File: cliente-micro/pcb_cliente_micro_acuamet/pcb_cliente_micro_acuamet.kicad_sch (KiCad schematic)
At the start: 43 parts, among them J1 Presion, J10 5V IN, J11 Botones, J2 Ultrasonico, J3 Valvula 1, J4 Valvula 2, J5 Relay, J6 Debug, J7 Valvula 3, J8 LCD, J9 Valvula 4, U1 M7, U2 M7, U3 AMS1117-3.3_C347222, U4 ESP32-WROOM-32D

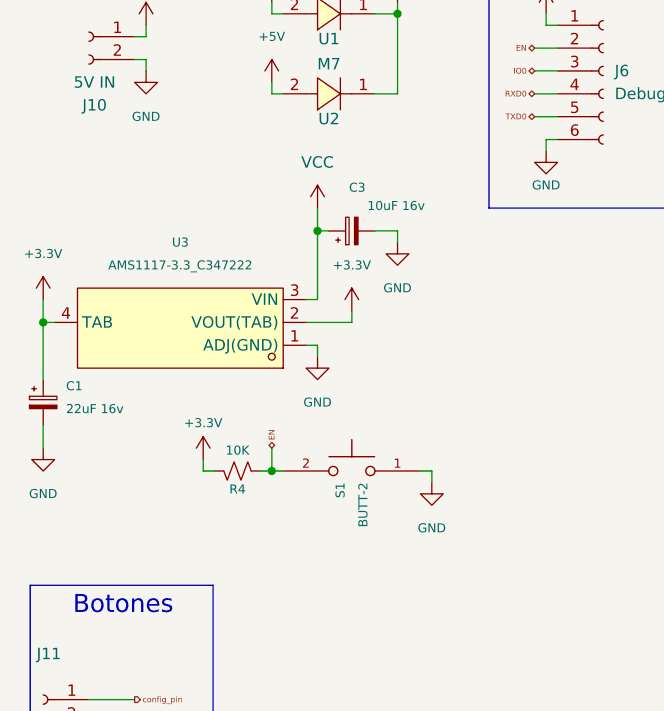
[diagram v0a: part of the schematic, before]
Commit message: Version final PCB
Version revisada y corregida
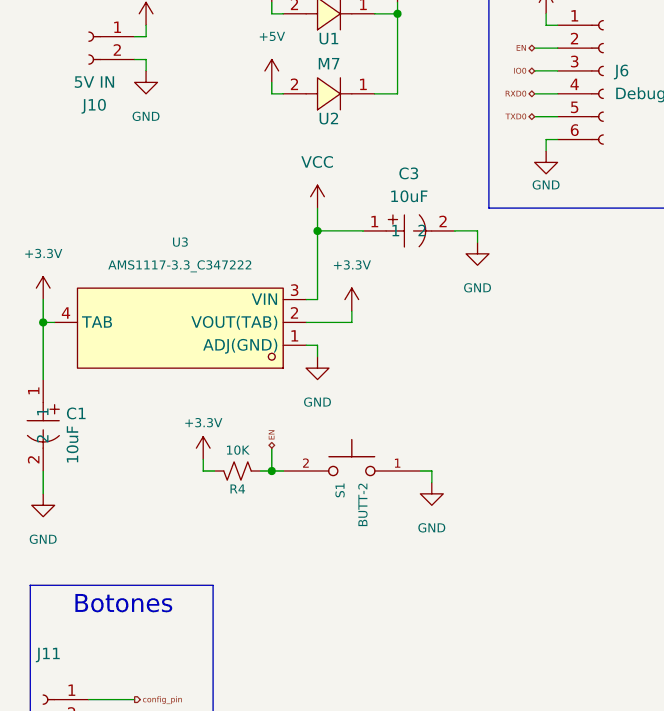
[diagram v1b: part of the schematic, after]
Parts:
- removed C1: 22uF 16v, Capacitor_THT:CP_Radial_D6.3mm_P2.50mm, symbol Device:C_Polarized_Small
- removed C3: 10uF 16v, Capacitor_THT:CP_Radial_D6.3mm_P2.50mm, symbol Device:C_Polarized_Small
- added C1, C3: 10uF, EasyEDA:CAP-SMD_L3.2-W1.6, symbol EasyEDA:TMCMA1C106KTRF
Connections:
- net +3.3V: now also C1.1
- net GND: now also C1.2, C3.2
- net VCC: now also C3.1
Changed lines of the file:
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@@
 	(wire
 		(pts
-			(xy 54.61 46.99) (xy 57.15 46.99)
+			(xy 63.5 46.99) (xy 66.04 46.99)
 		)
 		(stroke
@@
 	(wire
 		(pts
-			(xy 57.15 46.99) (xy 57.15 48.26)
+			(xy 66.04 46.99) (xy 66.04 48.26)
 		)
 		(stroke
@@
 	(wire
 		(pts
+			(xy 17.78 73.66) (xy 17.78 76.2)
+		)
+		(stroke
+			(width 0)
+			(type default)
+		)
+	)
+	(wire
+		(pts
 			(xy 91.44 26.67) (xy 91.44 25.4)
 		)
@@
 	(wire
 		(pts
-			(xy 17.78 68.58) (xy 17.78 71.12)
-		)
-		(stroke
-			(width 0)
-			(type default)
-		)
-	)
-	(wire
-		(pts
 			(xy 139.7 163.83) (xy 143.51 163.83)
 		)
@@
 	(wire
 		(pts
-			(xy 48.26 46.99) (xy 49.53 46.99)
+			(xy 48.26 46.99) (xy 53.34 46.99)
 		)
 		(stroke
@@
 	(symbol
 		(lib_id "power:GND")
-		(at 57.15 48.26 0)
+		(at 66.04 48.26 0)
 		(unit 1)
 		(exclude_from_sim no)
@@
 		(fields_autoplaced yes)
 		(property "Reference" "#PWR023"
-			(at 57.15 54.61 0)
+			(at 66.04 54.61 0)
 			(effects
 				(font
@@
 		)
 		(property "Value" "GND"
-			(at 57.15 53.34 0)
+			(at 66.04 53.34 0)
 			(effects
 				(font
@@
 		)
 		(property "Footprint" ""
-			(at 57.15 48.26 0)
+			(at 66.04 48.26 0)
 			(effects
 				(font
@@
 		)
 		(property "Datasheet" ""
-			(at 57.15 48.26 0)
+			(at 66.04 48.26 0)
 			(effects
 				(font
@@
 		)
 		(property "Description" "Power symbol creates a global label with name \"GND\" , ground"
-			(at 57.15 48.26 0)
+			(at 66.04 48.26 0)
 			(effects
 				(font
@@
 	)
 	(symbol
-		(lib_id "Device:C_Polarized_Small")
-		(at 52.07 46.99 90)
-		(unit 1)
-		(exclude_from_sim no)
-		(in_bom yes)
-		(on_board yes)
-		(dnp no)
-		(property "Reference" "C3"
-			(at 53.594 42.164 90)
-			(effects
-				(font
-					(size 1 1)
-				)
-				(justify left)
-			)
-		)
-		(property "Value" "10uF 16v"
-			(at 60.198 44.196 90)
-			(effects
-				(font
-					(size 1 1)
-				)
-				(justify left)
-			)
-		)
-		(property "Footprint" "Capacitor_THT:CP_Radial_D6.3mm_P2.50mm"
-			(at 52.07 46.99 0)
-			(effects
-				(font
-					(size 1.27 1.27)
-				)
-				(hide yes)
-			)
-		)
-		(property "Datasheet" "~"
-			(at 52.07 46.99 0)
-			(effects
-				(font
-					(size 1.27 1.27)
-				)
-				(hide yes)
-			)
-		)
-		(property "Description" "Polarized capacitor, small symbol"
-			(at 52.07 46.99 0)
-			(effects
-				(font
-					(size 1.27 1.27)
-				)
-				(hide yes)
-			)
-		)
-		(pin "1"
-		)
-		(pin "2"
-		)
-		(instances
-			(project ""
-				(path "/40156f8c-40d9-435e-851b-9df8dfaedb63"
-					(reference "C3")
-					(unit 1)
-				)
-			)
-		)
-	)
-	(symbol
 		(lib_id "power:+5V")
 		(at 43.18 30.48 0)
@@
 	(symbol
 		(lib_id "power:GND")
-		(at 17.78 71.12 0)
+		(at 17.78 76.2 0)
 		(unit 1)
 		(exclude_from_sim no)
@@
 		(fields_autoplaced yes)
 		(property "Reference" "#PWR04"
-			(at 17.78 77.47 0)
+			(at 17.78 82.55 0)
 			(effects
 				(font
@@
 		)
 		(property "Value" "GND"
-			(at 17.78 76.2 0)
+			(at 17.78 81.28 0)
 			(effects
 				(font
@@
 		)
 		(property "Footprint" ""
-			(at 17.78 71.12 0)
+			(at 17.78 76.2 0)
 			(effects
 				(font
@@
 		)
 		(property "Datasheet" ""
-			(at 17.78 71.12 0)
+			(at 17.78 76.2 0)
 			(effects
 				(font
@@
 		)
 		(property "Description" "Power symbol creates a global label with name \"GND\" , ground"
-			(at 17.78 71.12 0)
+			(at 17.78 76.2 0)
 			(effects
 				(font
@@
 	)
 	(symbol
+		(lib_id "EasyEDA:TMCMA1C106KTRF")
+		(at 156.21 123.19 0)
+		(unit 1)
+		(exclude_from_sim no)
+		(in_bom yes)
+		(on_board yes)
+		(dnp no)
+		(fields_autoplaced yes)
+		(property "Reference" "C3"
+			(at 58.42 40.64 0)
+			(effects
+				(font
+					(size 1.27 1.27)
+				)
+			)
+		)
+		(property "Value" "10uF"
+			(at 58.42 43.18 0)
+			(effects
+				(font
+					(size 1.27 1.27)
+				)
+			)
+		)
+		(property "Footprint" "EasyEDA:CAP-SMD_L3.2-W1.6"
+			(at 156.21 54.61 0)
+			(effects
+				(font
+					(size 1.27 1.27)
+				)
+				(hide yes)
+			)
+		)
+		(property "Datasheet" ""
+			(at 156.21 123.19 0)
+			(effects
+				(font
+					(size 1.27 1.27)
+				)
+				(hide yes)
+			)
+		)
+		(property "Description" ""
+			(at 156.21 123.19 0)
+			(effects
+				(font
+					(size 1.27 1.27)
+				)
+				(hide yes)
+			)
+		)
+		(property "LCSC Part" "C4988312"
+			(at 156.21 57.15 0)
+			(effects
+				(font
+					(size 1.27 1.27)
+				)
+				(hide yes)
+			)
+		)
+		(pin "1"
+		)
+		(pin "2"
+		)
+		(instances
+			(project ""
+				(path "/40156f8c-40d9-435e-851b-9df8dfaedb63"
+					(reference "C3")
+					(unit 1)
+				)
+			)
+		)
+	)
+	(symbol
 		(lib_id "Device:R_Small_US")
 		(at 137.16 171.45 90)
@@
 	)
 	(symbol
+		(lib_name "TMCMA1C106KTRF_1")
+		(lib_id "EasyEDA:TMCMA1C106KTRF")
+		(at 17.78 68.58 270)
+		(unit 1)
+		(exclude_from_sim no)
+		(in_bom yes)
+		(on_board yes)
+		(dnp no)
+		(property "Reference" "C1"
+			(at 20.32 67.3099 90)
+			(effects
+				(font
+					(size 1.27 1.27)
+				)
+				(justify left)
+			)
+		)
+		(property "Value" "10uF"
+			(at 21.082 68.58 0)
+			(effects
+				(font
+					(size 1.27 1.27)
+				)
+				(justify left)
+			)
+		)
+		(property "Footprint" "EasyEDA:CAP-SMD_L3.2-W1.6"
+			(at 29.464 69.342 0)
+			(effects
+				(font
+					(size 1.27 1.27)
+				)
+				(hide yes)
+			)
+		)
+		(property "Datasheet" ""
+			(at 17.78 68.58 0)
+			(effects
+				(font
+					(size 1.27 1.27)
+				)
+				(hide yes)
+			)
+		)
+		(property "Description" ""
+			(at 17.78 68.58 0)
+			(effects
+				(font
+					(size 1.27 1.27)
+				)
+				(hide yes)
+			)
+		)
+		(property "LCSC Part" "C4988312"
+			(at 26.924 69.342 0)
+			(effects
+				(font
+					(size 1.27 1.27)
+				)
+				(hide yes)
+			)
+		)
+		(pin "1"
+		)
+		(pin "2"
+		)
+		(instances
+			(project "pcb_cliente_micro_acuamet"
+				(path "/40156f8c-40d9-435e-851b-9df8dfaedb63"
+					(reference "C1")
+					(unit 1)
+				)
+			)
+		)
+	)
+	(symbol
 		(lib_id "Device:C_Small")
 		(at 50.8808 154.6407 180)
@@
 					(unit 1)
 				)
-			)
-		)
-	)
-	(symbol
-		(lib_id "Device:C_Polarized_Small")
-		(at 17.78 66.04 0)
-		(unit 1)
-		(exclude_from_sim no)
-		(in_bom yes)
-		(on_board yes)
-		(dnp no)
-		(fields_autoplaced yes)
-		(property "Reference" "C1"
-			(at 20.32 64.2238 0)
-			(effects
-				(font
-					(size 1 1)
-				)
-				(justify left)
-			)
-		)
-		(property "Value" "22uF 16v"
-			(at 20.32 66.7638 0)
-			(effects
-				(font
-					(size 1 1)
-				)
-				(justify left)
-			)
-		)
-		(property "Footprint" "Capacitor_THT:CP_Radial_D6.3mm_P2.50mm"
-			(at 17.78 66.04 0)
-			(effects
-				(font
-					(size 1.27 1.27)
-				)
-				(hide yes)
-			)
-		)
-		(property "Datasheet" "~"
-			(at 17.78 66.04 0)
-			(effects
-				(font
-					(size 1.27 1.27)
-				)
-				(hide yes)
-			)
-		)
-		(property "Description" "Polarized capacitor, small symbol"
-			(at 17.78 66.04 0)
-			(effects
-				(font
-					(size 1.27 1.27)
-				)
-				(hide yes)
-			)
-		)
-		(pin "1"
-		)
-		(pin "2"
-		)
-		(instances
-			(project "pcb_cliente_micro_acuamet"
-				(path "/40156f8c-40d9-435e-851b-9df8dfaedb63"
-					(reference "C1")
-					(unit 1)
-				)
